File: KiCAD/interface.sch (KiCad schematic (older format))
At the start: 32 parts, among them P10 C3SB, P11 VSel_Vlv, P14 X_VALVE, P17 PUMP, P18 Pump_Cable, P34 VSel_Vlv2, P38 X_VALVE2, P7 GAGE_PR, P9 C3SB, Q1 BCP5416TA, Q2 BCP5416TA, Q3 BCP5416TA, Q4 BCP5416TA, U1 TXB0104D

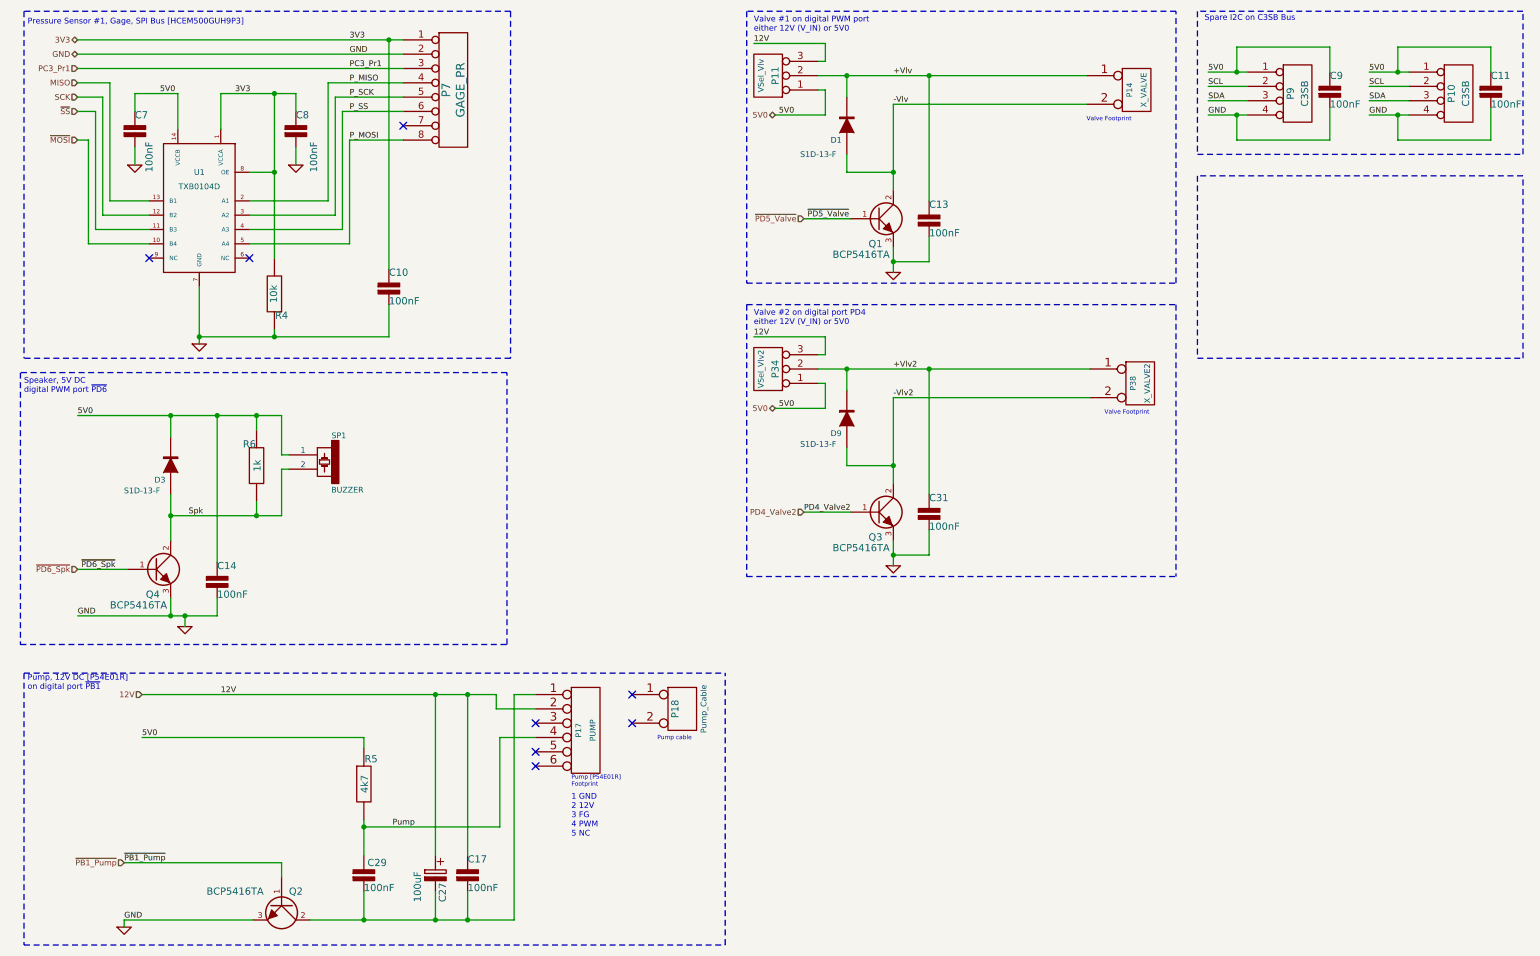
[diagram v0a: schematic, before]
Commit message: layout, work in progress
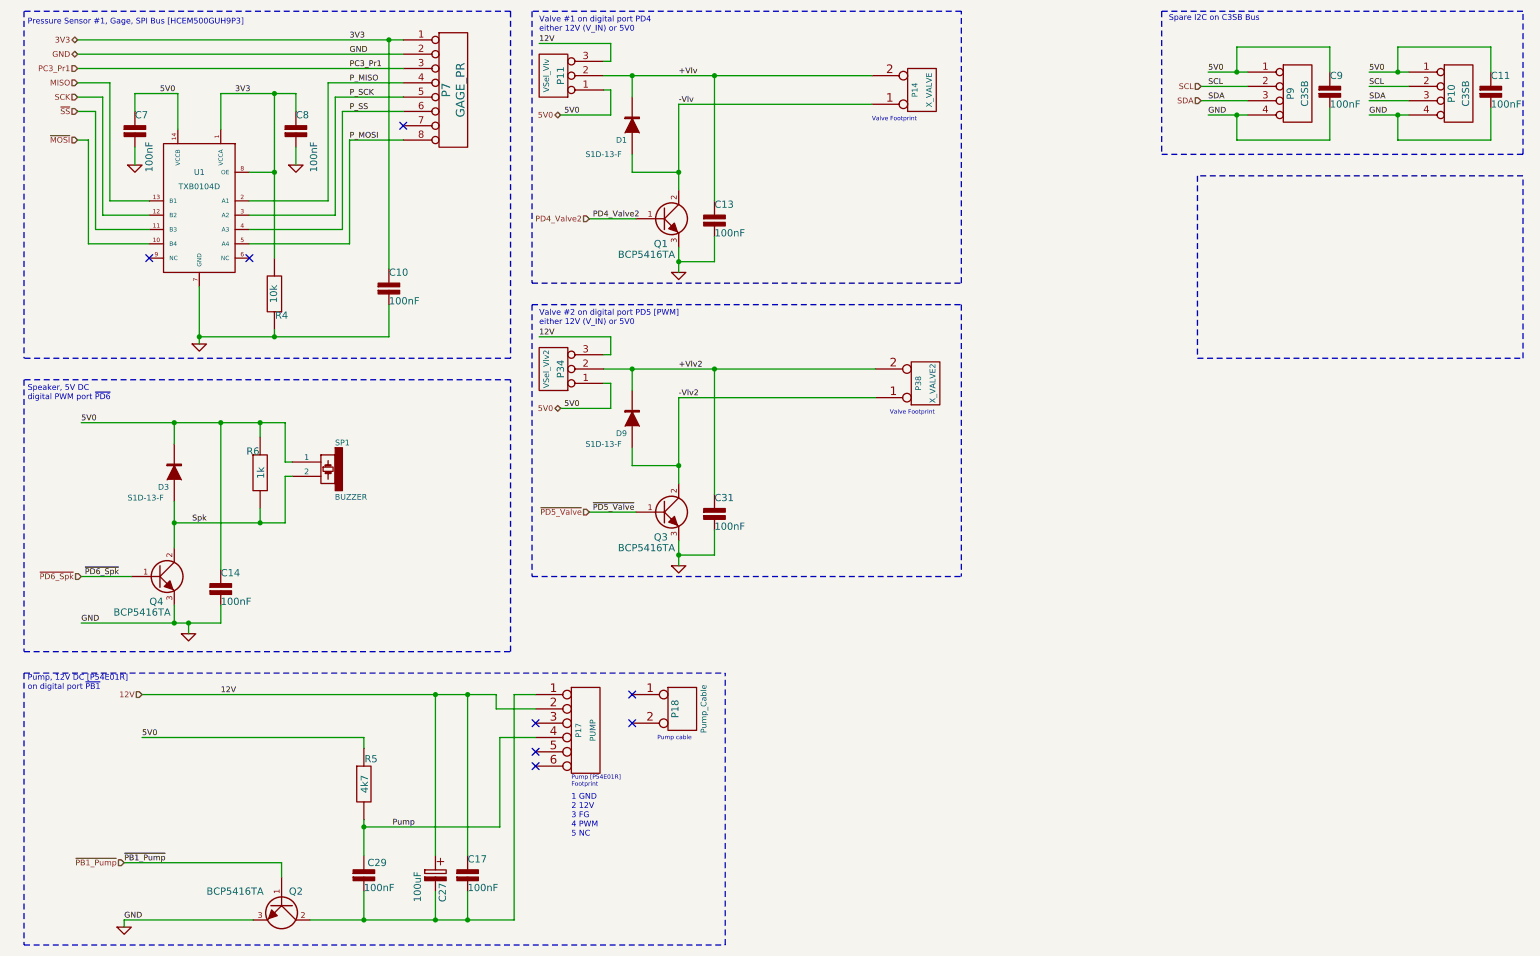
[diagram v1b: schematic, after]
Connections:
- net +Vlv: now also P14.2 (PM); no longer P14.1 (P1)
- net +Vlv2: now also P38.2 (PM); no longer P38.1 (P1)
- net -Vlv: now also P14.1 (P1); no longer P14.2 (PM)
- net -Vlv2: now also P38.1 (P1); no longer P38.2 (PM)
- net PD4_Valve2: now also Q1.1 (B); no longer Q3.1 (B)
- net ~PD5_Valve: now also Q3.1 (B); no longer Q1.1 (B)
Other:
- note added: "Valve #1 on digital port PD4\neither 12V (V_IN) or 5V0"
- note added: "Valve #2 on digital port PD5 [PWM]\neither 12V (V_IN) or 5V0"
- note removed: "Valve #1 on digital PWM port\neither 12V (V_IN) or 5V0"
- note removed: "Valve #2 on digital port PD4\neither 12V (V_IN) or 5V0"
- moved on the sheet: C13, C14, C31, D1, D3, D9, P11, P14, P34, P38, Q1, Q3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
